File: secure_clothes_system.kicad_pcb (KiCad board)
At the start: 4 copper layers, 28 x 33.9 mm, 32 parts, among them J1 UART0, SW1 BOOT, SW2 RST, U1 TPS62842DGRR, U2 ESP32-C3, U3 W25X40CLSN, Y1 40MHz

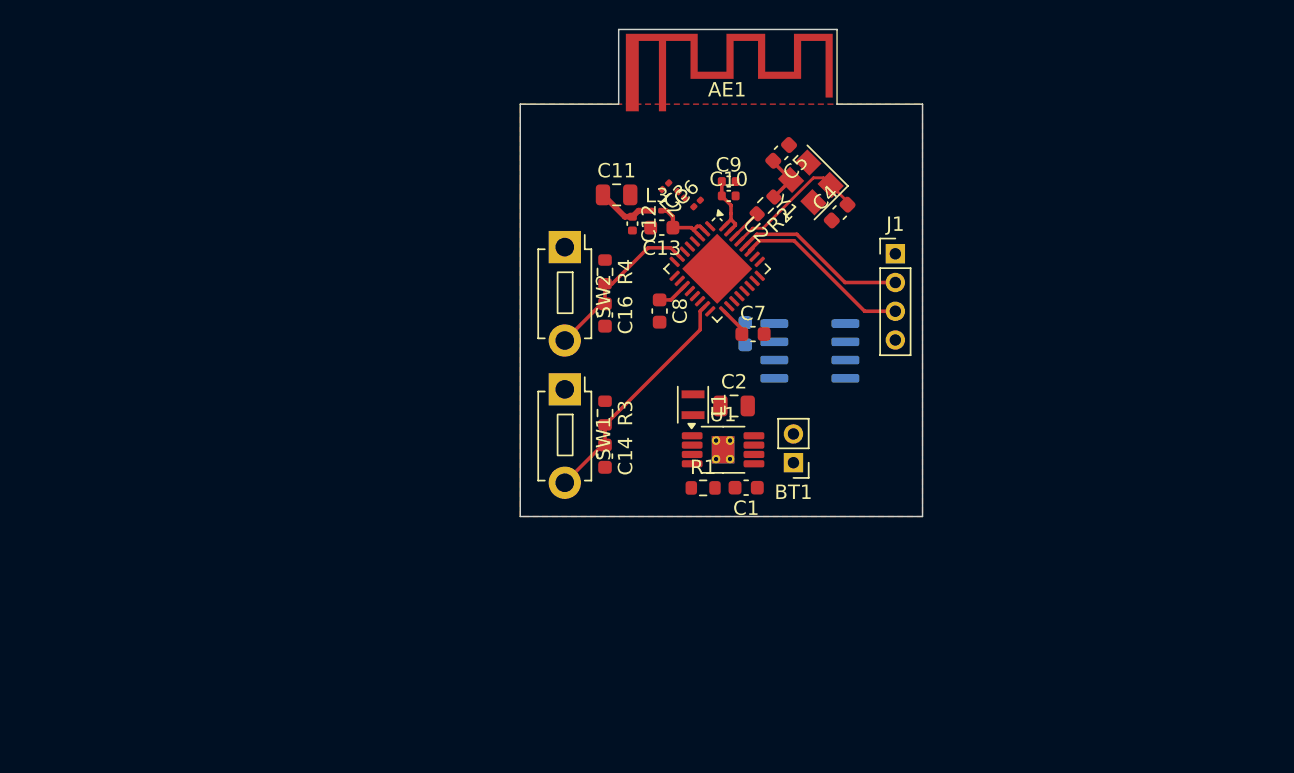
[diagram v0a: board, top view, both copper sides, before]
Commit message: Made some fixes with the layout
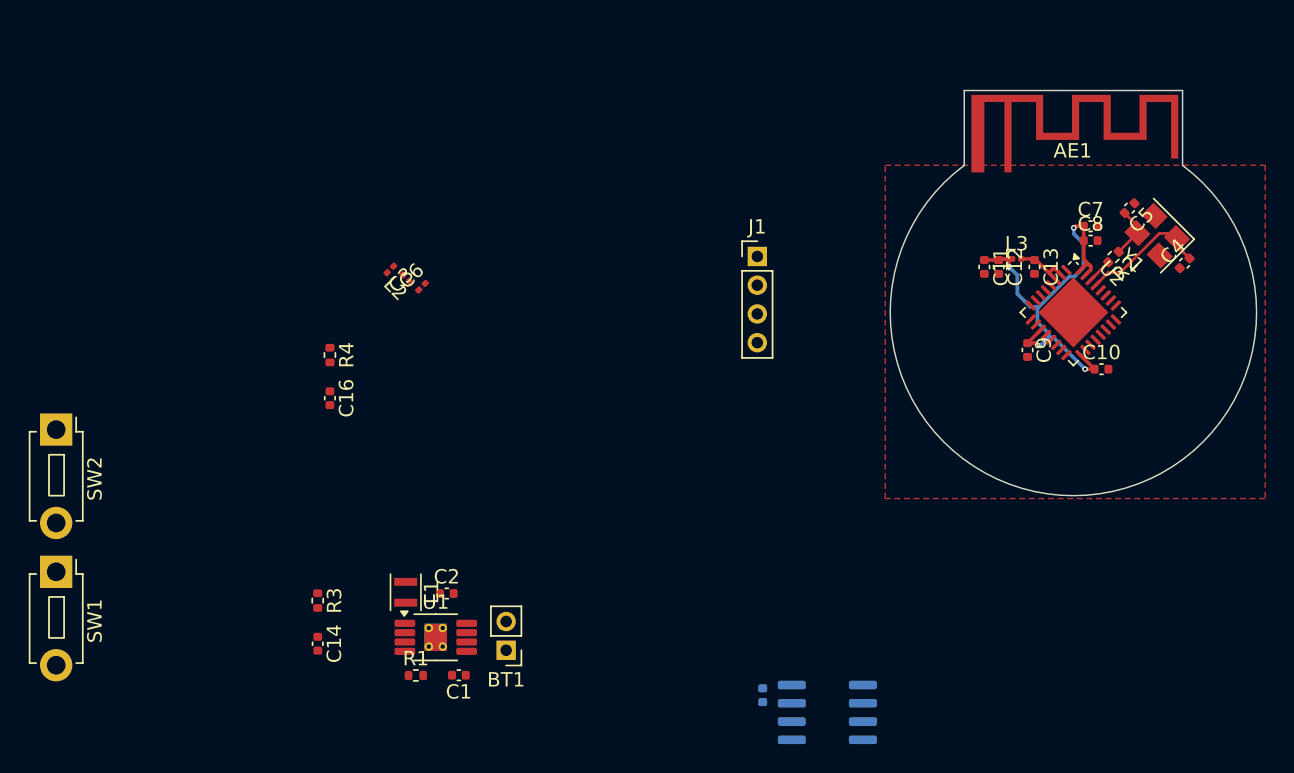
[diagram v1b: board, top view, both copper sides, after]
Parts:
- C1, C13, C14, C15, C16, C4, C5, C7, C8: footprint Capacitor_SMD:C_0603_1608Metric -> Capacitor_SMD:C_0402_1005Metric
- C11, C2: footprint Capacitor_SMD:C_0805_2012Metric -> Capacitor_SMD:C_0402_1005Metric
- R1: value 267K -> 52.3K; footprint Resistor_SMD:R_0603_1608Metric -> Resistor_SMD:R_0402_1005Metric
- R2, R3, R4: footprint Resistor_SMD:R_0603_1608Metric -> Resistor_SMD:R_0402_1005Metric
- moved SW1 37.6 mm to (104.7, 108.0)
- moved SW2 37.6 mm to (104.7, 98.2)
- moved C8 30.4 mm to (176.7, 85.0), turned to 0 degrees
- moved C10 28.6 mm to (177.5, 93.9)
- moved C13 26.1 mm to (172.8, 86.8), turned to -90 degrees
- moved C11 26.1 mm to (169.3, 86.8), turned to -90 degrees
- moved C12 25.7 mm to (170.3, 86.8)
- moved L3 25.3 mm to (171.5, 86.3)
- moved C15 25.2 mm to (153.9, 116.6)
- moved U3 25.2 mm to (158.4, 117.8)
- moved U2 25.0 mm to (175.5, 90.0)
- moved C7 24.7 mm to (176.7, 84.0)
- moved C5 24.6 mm to (179.4, 82.7)
- moved R2 24.5 mm to (178.3, 86.1)
- moved AE1 24.4 mm to (170.9, 80.2)
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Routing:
- net +3V3: track 13.2 -> 30.6 mm, vias 0 -> 4
- net /ESP32-C3/BOOT: track 16.4 -> 0.00 mm
- net /ESP32-C3/U0RXD: track 12.5 -> 0.00 mm
- net /ESP32-C3/U0TXD: track 12.2 -> 0.00 mm
- net /ESP32-C3/CHIP_EN: track 11.7 -> 0.00 mm
- net /ESP32-C3/XTAL_N: track 10.3 -> 9.05 mm
- net /ESP32-C3/VDD3P3: track 4.93 -> 4.24 mm
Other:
- board size 28 x 33.9 mm -> 25.5 x 28.2 mm
